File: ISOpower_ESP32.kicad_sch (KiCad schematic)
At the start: 16 parts, among them J2 ESP_GPIO_B, J3 ESPpin4-7, J4 SDI-SDO, J5 i2c Header, J6 ESP_GPIO_A [Make New Part & L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, J7 Bus_PCI_Express_x1, U1 ESP32-WROOM-32, U2 AMS1117-3.3

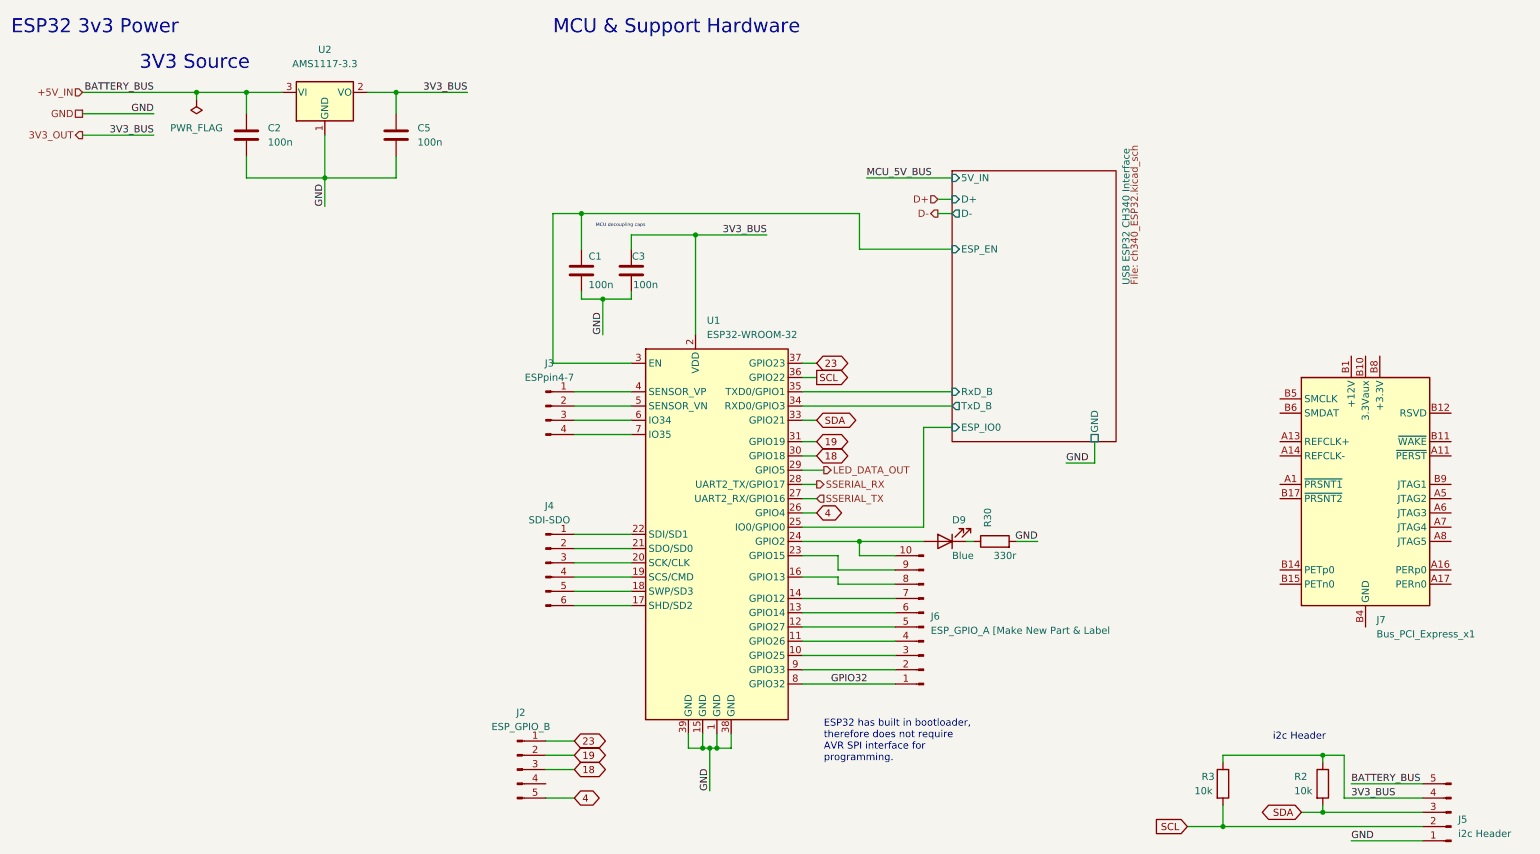
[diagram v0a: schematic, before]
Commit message: werewr
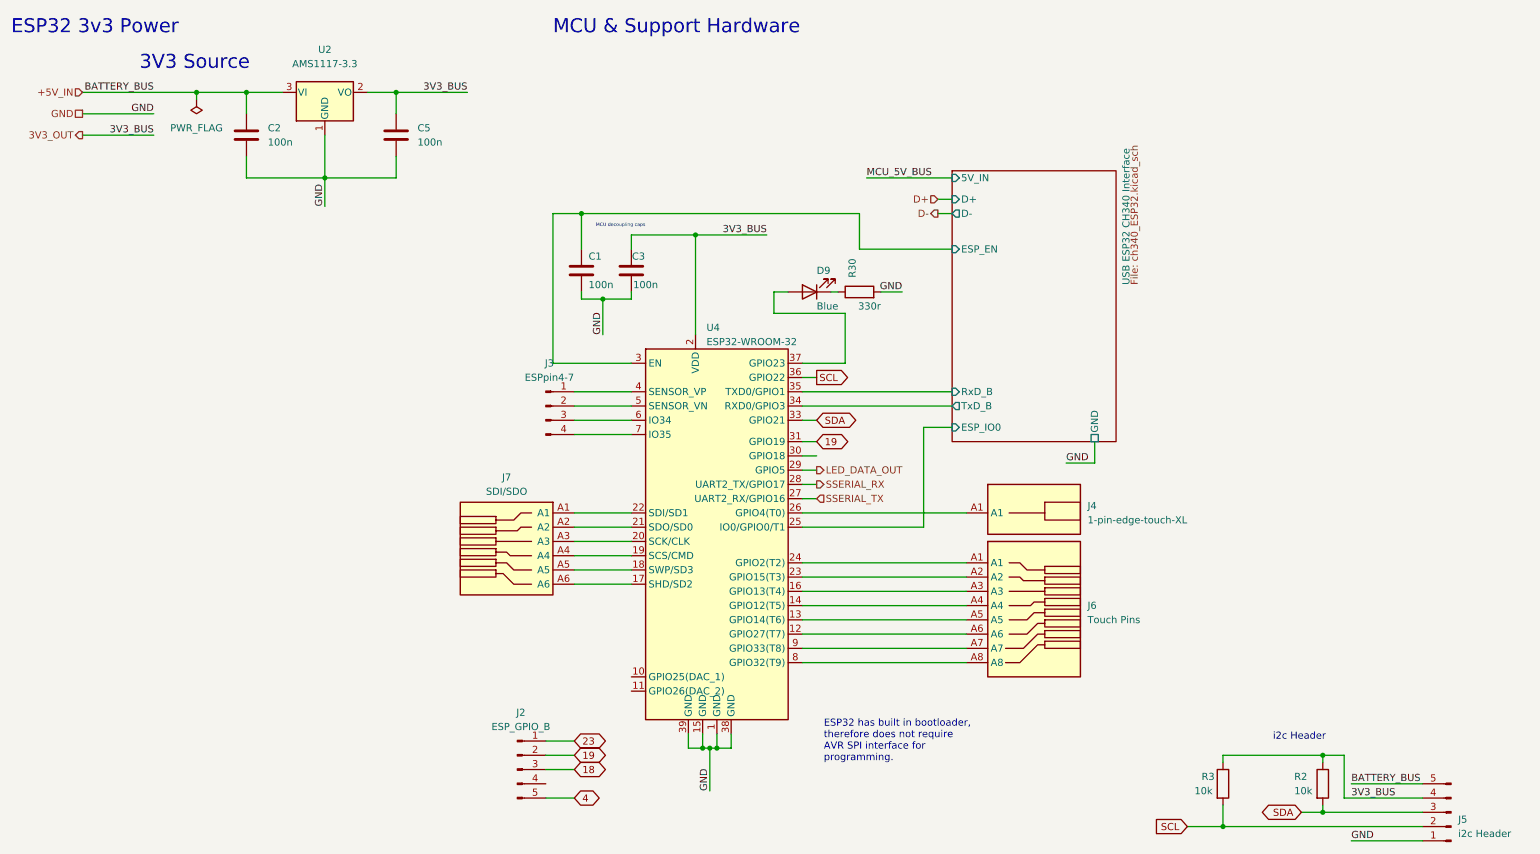
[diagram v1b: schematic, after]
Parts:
- removed J4: SDI-SDO, Connector_PinHeader_1.27mm:PinHeader_1x06_P1.27mm_Vertical, symbol Connector:Conn_01x06_Male
- removed J6: ESP_GPIO_A [Make New Part & Label, Connector_PinHeader_2.00mm:PinHeader_1x10_P2.00mm_Vertical, symbol 000_Pin_Headers_Immo:Conn_01x10_Pin
- removed J7: Bus_PCI_Express_x1, symbol Connector:Bus_PCI_Express_x1
- removed U1: ESP32-WROOM-32, RF_Module:ESP32-WROOM-32, symbol 000_MCU_microcontrollers_Immo:ESP32-WROOM-32
- added J4: 1-pin-edge-touch-XL, Connector_PCBEdge:BUS_PCIexpress_x1, symbol 000-edge-connectors-immo:1-pin-edge-touch-XL
- added J6: Touch Pins, Connector_PCBEdge:BUS_PCIexpress_x1, symbol 000-edge-connectors-immo:8-pin-edge-touch
- added J7: SDI/SDO, Connector_PCBEdge:BUS_PCIexpress_x1, symbol 000-edge-connectors-immo:6-pin-edge-touch
- added U4: ESP32-WROOM-32, RF_Module:ESP32-WROOM-32, symbol 000_MCU_microcontrollers_Immo:ESP32-WROOM-32_2
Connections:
- net 19: now also U4.31 (GPIO19)
- net 3V3_OUT: now also U4.2 (VDD)
- net GND: now also U4.1 (GND), U4.15 (GND), U4.38 (GND), U4.39 (GND)
- net LED_DATA_OUT: now also U4.29 (GPIO5)
- net SCL: now also U4.36 (GPIO22)
- net SDA: now also U4.33 (GPIO21)
- net SSERIAL_RX: now also U4.28 (UART2_TX/GPIO17)
- net SSERIAL_TX: now also U4.27 (UART2_RX/GPIO16)
- net USB ESP32 CH340 Interface /ESP_EN: now also U4.3 (EN)
- net USB ESP32 CH340 Interface /ESP_IO0: now also U4.25 (IO0/GPIO0/T1)
- net USB ESP32 CH340 Interface /RxD_B: now also U4.35 (TXD0/GPIO1)
- net USB ESP32 CH340 Interface /TxD_B: now also U4.34 (RXD0/GPIO3)
- net at D9.2 (A): now also U4.37 (GPIO23)
- net at J3.1 (Pin_1): now also U4.4 (SENSOR_VP)
- net at J3.2 (Pin_2): now also U4.5 (SENSOR_VN)
- net at J3.3 (Pin_3): now also U4.6 (IO34)
- net at J3.4 (Pin_4): now also U4.7 (IO35)
- new net: J4.A1, U4.26 (GPIO4(T0))
- new net: J6.A6, U4.12 (GPIO27(T7))
- new net: J6.A5, U4.13 (GPIO14(T6))
- new net: J6.A4, U4.14 (GPIO12(T5))
- new net: J6.A3, U4.16 (GPIO13(T4))
- new net: J7.A6, U4.17 (SHD/SD2)
- new net: J7.A5, U4.18 (SWP/SD3)
- new net: J7.A4, U4.19 (SCS/CMD)
- new net: J7.A3, U4.20 (SCK/CLK)
- new net: J7.A2, U4.21 (SDO/SD0)
- new net: J7.A1, U4.22 (SDI/SD1)
- new net: J6.A2, U4.23 (GPIO15(T3))
- new net: J6.A1, U4.24 (GPIO2(T2))
- new net: J6.A8, U4.8 (GPIO32(T9))
- new net: J6.A7, U4.9 (GPIO33(T8))
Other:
- moved on the sheet: D9, R30
